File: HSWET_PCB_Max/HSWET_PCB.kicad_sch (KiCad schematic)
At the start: 30 parts, among them IC3 PS2565L-1-V-F3-A, IC4 PS2565L-1-V-F3-A, IC5 PS2565L-1-V-F3-A, J1 CON-SOCJ-2155, J10 arduino enc, J11 turbine pwr, J2 emergency stop, J3 CON-SOCJ-2155, J4 turbine bus, J5 5v, J6 9v, J7 4.5v, J8 GND, J9 arduino lin act, U1 INA260AIPWR, U3 YAAJ_DCDC_StepDown_LM2596

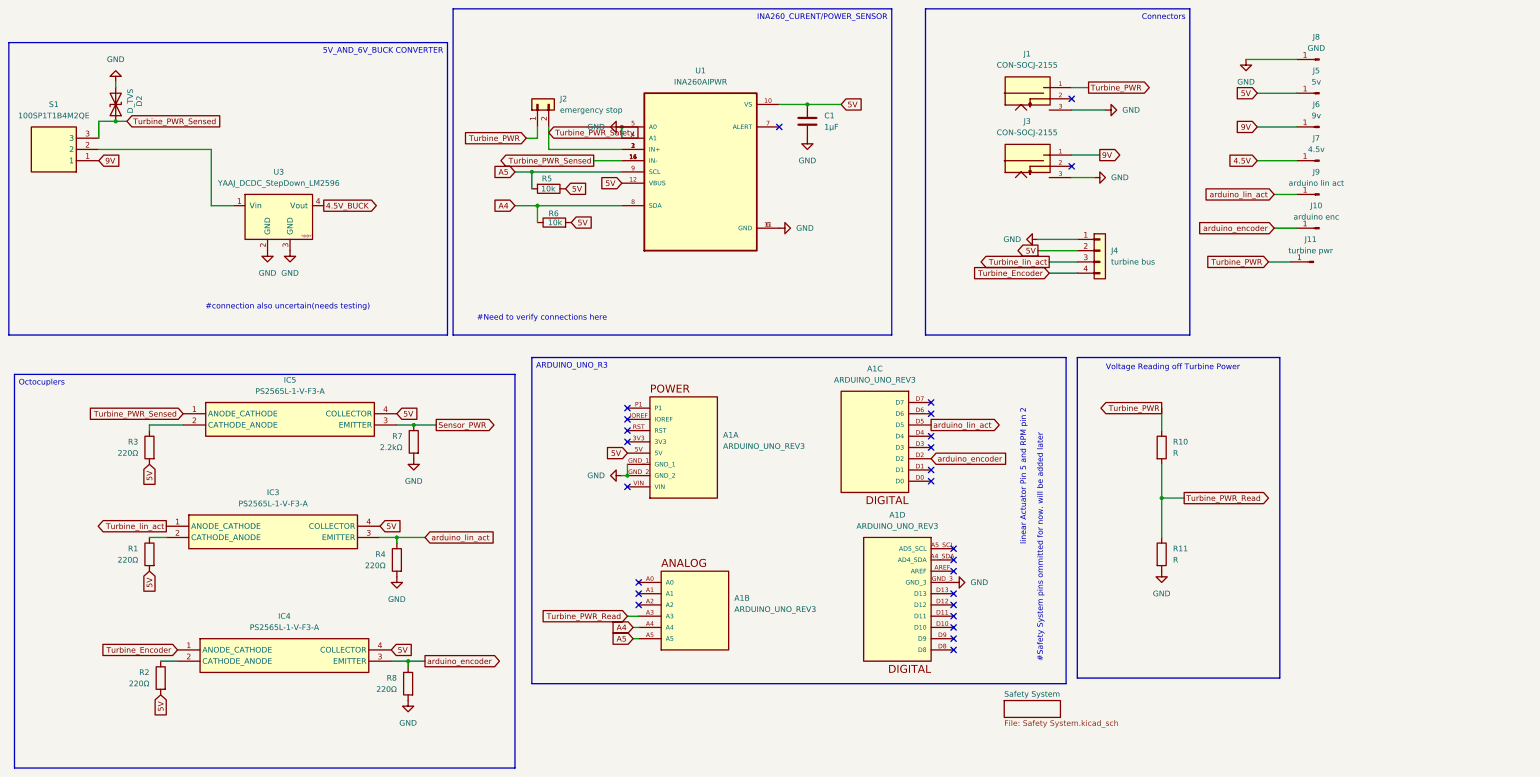
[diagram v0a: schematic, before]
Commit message: bruh
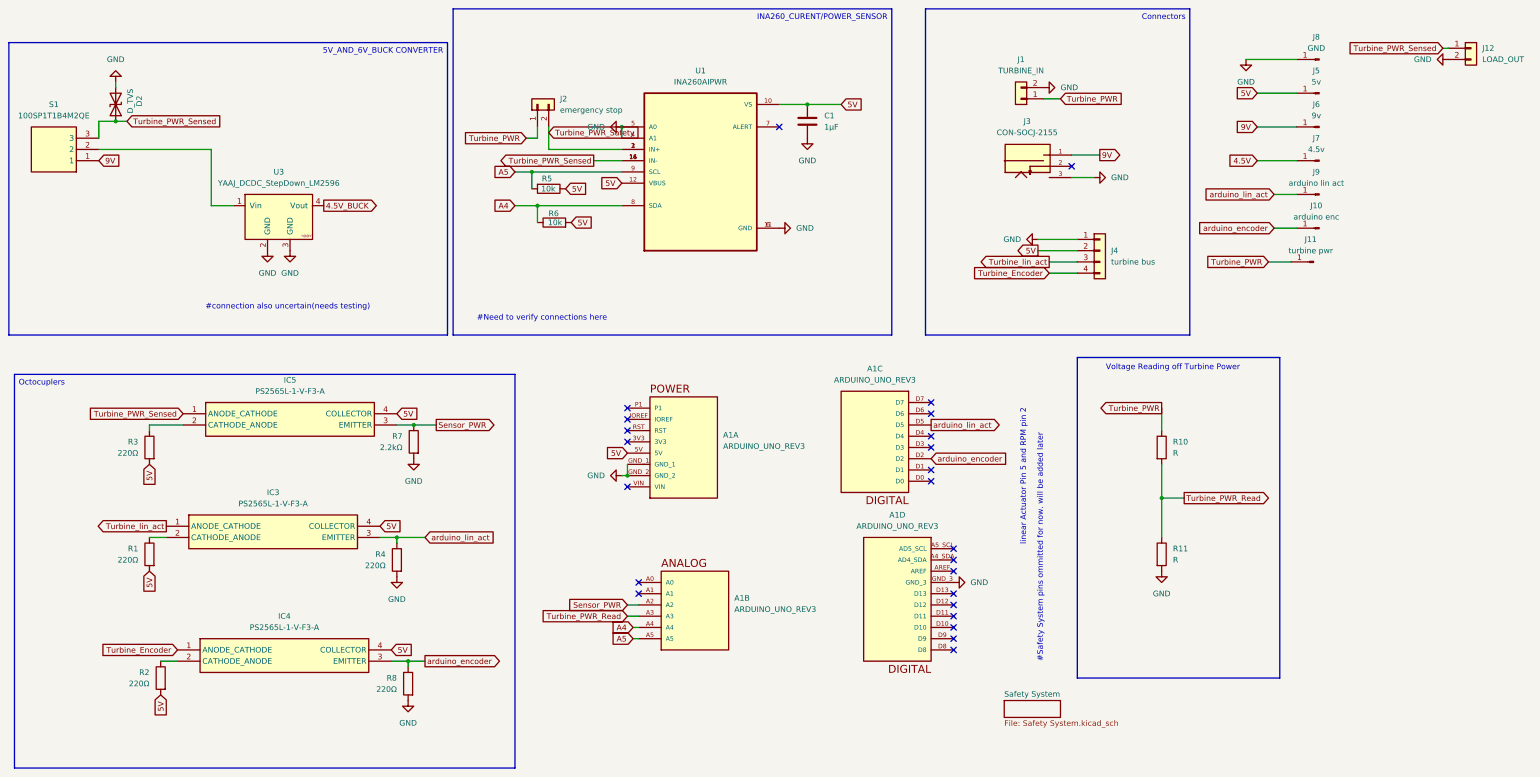
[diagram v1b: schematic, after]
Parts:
- removed J1: CON-SOCJ-2155, footprints:GRAVITECH_CON-SOCJ-2155, symbol CON-SOCJ-2155:CON-SOCJ-2155
- added J1: TURBINE_IN, Connector_AMASS:AMASS_XT30PW-M_1x02_P2.50mm_Horizontal, symbol Connector_Generic:Conn_01x02
- added J12: LOAD_OUT, Connector_AMASS:AMASS_XT30PW-M_1x02_P2.50mm_Horizontal, symbol Connector_Generic:Conn_01x02
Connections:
- net GND: now also J1.2 (Pin_2), J12.2 (Pin_2)
- net Sensor_PWR: now also A1.A2
- net Turbine_PWR: now also J1.1 (Pin_1)
- net Turbine_PWR_Sensed: now also J12.1 (Pin_1)
- no-connect marks 26 -> 24
